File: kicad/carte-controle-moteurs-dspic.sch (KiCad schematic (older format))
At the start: 73 parts, among them P1 GND, P10 CONN_1, P11 ALIM, P12 MOTEUR 1, P13 MOTEUR 2, P14 PILES, P15 PILES, P17 I2C, P18 ENCODEUR 1, P19 ENCODEUR 2, P2 5V, P20 PROG, P21 Fixe, P22 Fixe, P23 Fixe, P24 Fixe, P3 3.3V, P4 EN, P5 L1, P6 H1, P7 L2, P8 H2, P9 CONN_1, U1 DSPIC33FJ, U2 L298_PAI225, U3 LM1117-3.3, X1 10 MHz

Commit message: Mise à jour des fichiers pour la nouvelle version de KiCAD
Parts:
- removed C10: 17p, symbol C
- removed C11, C12, C13: 1u, symbol CAPAPOL
- removed C14: 4.7u, symbol CAPAPOL
- removed C2, C3, C4: 100n, symbol C
- removed C6, C7, C8: 100u, symbol CAPAPOL
- removed D1, D10, D2, D3, D4, D5, D6, D7, D8, D9: 5A, symbol DIODE
- removed D11, D12: GREEN, symbol LED
- removed D13: RED, symbol LED
- removed D14, D15, D16, D17, D18, D19: ZENER, symbol DIODE
- removed P1: GND, symbol CONN_1
- removed P10, P9: CONN_1, symbol CONN_1
- removed P11: ALIM, symbol CONN_2
- removed P12: MOTEUR 1, symbol CONN_2
- removed P13: MOTEUR 2, symbol CONN_2
- removed P14, P15: PILES, symbol CONN_2
- removed P17: I2C, symbol CONN_4
- removed P18: ENCODEUR 1, symbol CONN_5
- removed P19: ENCODEUR 2, symbol CONN_5
- removed P2: 5V, symbol CONN_1
- removed P20: PROG, symbol CONN_5X2
- removed P21, P22, P23, P24: Fixe, symbol CONN_1
- removed P3: 3.3V, symbol CONN_1
- removed P4: EN, symbol CONN_1
- removed P5: L1, symbol CONN_1
- removed P6: H1, symbol CONN_1
- removed P7: L2, symbol CONN_1
- removed P8: H2, symbol CONN_1
- removed U3: LM1117-3.3, symbol LM317T
- removed X1: 10 MHz, symbol CRYSTAL
- added C10, C2, C3, C4, C7: 100u, Capacitors_THT:CP_Radial_D10.0mm_P2.50mm_P5.00mm, symbol CP
- added C11, C12: 17p, Capacitors_THT:C_Rect_L7.0mm_W3.5mm_P2.50mm_P5.00mm, symbol C
- added C13: 1u, Capacitors_THT:CP_Radial_D10.0mm_P2.50mm_P5.00mm, symbol CP
- added C14: 4.7u, Capacitors_THT:CP_Radial_D10.0mm_P2.50mm_P5.00mm, symbol CP
- added C6, C8: 100n, Capacitors_THT:C_Rect_L7.0mm_W3.5mm_P2.50mm_P5.00mm, symbol C
- added D1: RED, LEDs:LED_D3.0mm, symbol LED
- added D10, D11, D12, D3, D4, D5, D6, D7, D8, D9: 5A, Diodes_THT:D_A-405_P10.16mm_Horizontal, symbol D
- added D13, D14, D15, D16, D17, D18: 3A, Diodes_THT:D_A-405_P10.16mm_Horizontal, symbol D_Zener
- added D19: GREEN, LEDs:LED_D3.0mm, symbol LED
- added D2: ORANGE, LEDs:LED_D3.0mm, symbol LED
- added J1: PDB, Measurement_Points:Measurement_Point_Round-TH_Small, symbol Conn_01x01
- added J10: PWR_IN, Connectors_Molex:Molex_MiniFit-JR-5569-04A2_2x02x4.20mm_Angled, symbol Conn_02x02_Odd_Even
- added J11: GND, Measurement_Points:Measurement_Point_Round-TH_Small, symbol Conn_01x01
- added J12: 5V, Measurement_Points:Measurement_Point_Round-TH_Small, symbol Conn_01x01
- added J13: 3.3V, Measurement_Points:Measurement_Point_Round-TH_Small, symbol Conn_01x01
- added J14: EN, Measurement_Points:Measurement_Point_Round-TH_Small, symbol Conn_01x01
- added J15: MOTEUR 1, epsa_connect:KK_2C, symbol Conn_01x02
- added J16: MOTEUR 2, epsa_connect:KK_2C, symbol Conn_01x02
- added J17: L1, Measurement_Points:Measurement_Point_Round-TH_Small, symbol Conn_01x01
- added J18: H1, Measurement_Points:Measurement_Point_Round-TH_Small, symbol Conn_01x01
- added J19: L2, Measurement_Points:Measurement_Point_Round-TH_Small, symbol Conn_01x01
- added J2: I2C, epsa_connect:KK_4C, symbol Conn_01x04
- added J20: H2, Measurement_Points:Measurement_Point_Round-TH_Small, symbol Conn_01x01
- added J21: ENCODEUR 1, Pin_Headers:Pin_Header_Angled_1x05_Pitch2.54mm, symbol Conn_01x05
- added J22: RA1, Measurement_Points:Measurement_Point_Round-TH_Small, symbol Conn_01x01
- added J23: ENCODEUR 2, Pin_Headers:Pin_Header_Angled_1x05_Pitch2.54mm, symbol Conn_01x05
- added J3: PROG, Pin_Headers:Pin_Header_Angled_2x05_Pitch2.54mm, symbol Conn_02x05_Odd_Even
- added J4, J5: PILES, epsa_connect:KK_2C, symbol Conn_01x02
- added J6, J7, J8, J9: Fix, Connectors:1pin, symbol Conn_01x01
- added Y1: 10MHz, Crystals:Crystal_HC18-U_Vertical, symbol Crystal
- C1, C5: footprint (none) -> Capacitors_THT:C_Rect_L7.0mm_W3.5mm_P2.50mm_P5.00mm
- C9: value 17p -> 100n; footprint (none) -> Capacitors_THT:C_Rect_L7.0mm_W3.5mm_P2.50mm_P5.00mm
- R1, R12, R2, R5, R6, R7, R8: footprint (none) -> Resistors_THT:R_Axial_DIN0204_L3.6mm_D1.6mm_P2.54mm_Vertical
- R10, R11: value 470 -> 150; footprint (none) -> Resistors_THT:R_Axial_DIN0204_L3.6mm_D1.6mm_P2.54mm_Vertical
- R3: value 10 K -> 470; footprint (none) -> Resistors_THT:R_Axial_DIN0204_L3.6mm_D1.6mm_P2.54mm_Vertical
- R4: value 150 -> 470; footprint (none) -> Resistors_THT:R_Axial_DIN0204_L3.6mm_D1.6mm_P2.54mm_Vertical
- R9: value 150 -> 10K; footprint (none) -> Resistors_THT:R_Axial_DIN0204_L3.6mm_D1.6mm_P2.54mm_Vertical
- RR1: footprint (none) -> Resistors_THT:R_Array_SIP9
- U1: renamed from U2; footprint ANNEE 2017-2018 CONTACTER G. CHARREAUX -> TO_SOT_Packages_THT:Multiwatt-15_Vertical_StaggeredType1
- U2: renamed from U1; footprint (none) -> Housings_DIP:DIP-28_W7.62mm
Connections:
- net labels added: I2C_CLK, I2C_DATA, QEI1_CHA, QEI1_CHB, QEI2_CHA, QEI2_CHB
- net labels removed: I2C_clk, I2C_data, MCLR, QEI1_chA, QEI1_chB, QEI2_chA, QEI2_chB
- wire segments 179 -> 197
- no-connect marks 6 -> 7
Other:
- note added: "Connecteur d'alimentation"
- note added: "Convensions couleurs :\n1 - Noir : masse\n2 - Rouge : +5V\n3 - Orange : +3.3V\n4 - Jaune : BATT"
- note added: "DSPIC contrôle moteurs"
- note added: "Lissage tensions"
- note added: "Points de contrôle"
- note added: "Résistances de pull-up"
- note removed: "Branchement carte alim"
- note removed: "Connecteur I2C"
- note removed: "Connecteur de Programmation"
- note removed: "Conversion 5V-3.3V"
- note removed: "Dimensionner diodes (attention gros courant)"
- note removed: "Encodeurs moteurs"
- note removed: "Mettre infos en sérigraphie, pas en couche cuivre"
- note removed: "Need détrompeurs\nPlusieurs capas au lieu d'1 grosse"
- note removed: "PIC contrôle moteurs"
- note removed: "Pins de contrôle"
- note removed: "Pull up partagé i2c encodeur 20k réseau de résistance"
- note removed: "Rajouter diodes à endroits clés\n470 au lieu de 220"
- note removed: "Réseau de résistances - Pull up"
- note removed: "partir à la recherche de pdb"
- note removed: "pull up entre 10k et 100k en général 20k"
- note removed: "remplacer 18k par diodes zener"
- note removed: "vérifier si on a besoin du channel b des encodeurs (à priori non car ça sert pour la roue ibre)\nregrouper en1 et en2 (à voir)\nrb 10 et 11 utilisée pour debug (uart/rs232)"
- note removed: "zone à réserver sur le typon sans plan de masse pour puce d'identification"
- moved on the sheet: RR1, U1, U2

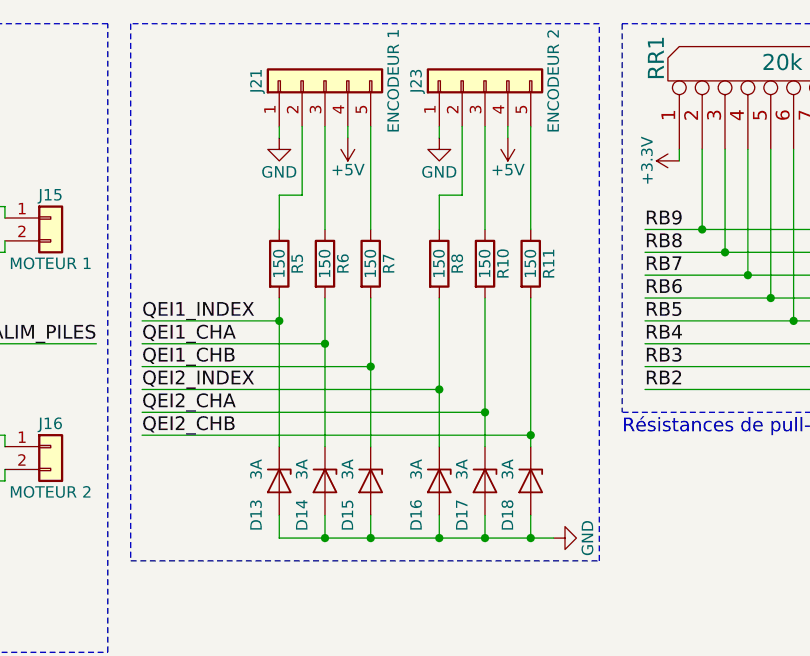
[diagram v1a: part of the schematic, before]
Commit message: Pré-validation CAO KiCAD
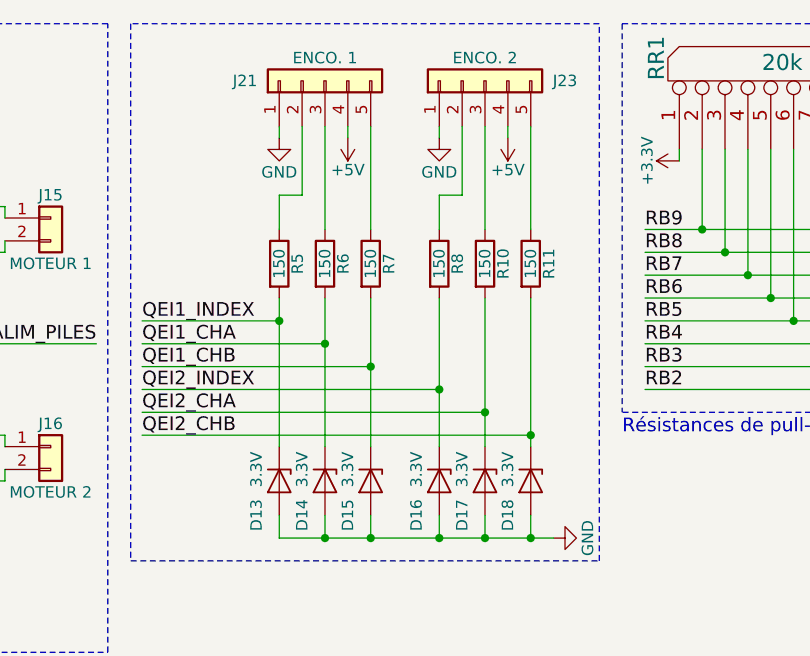
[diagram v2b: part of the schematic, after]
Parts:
- D13, D14, D15, D16, D17, D18: value 3A -> 3.3V
- J15, J16, J4, J5: footprint epsa_connect:KK_2C -> Connectors_Molex:Molex_MiniFit-JR-5569-02A2_2x01x4.20mm_Angled
- J21: value ENCODEUR 1 -> ENCO. 1
- J23: value ENCODEUR 2 -> ENCO. 2
- J3: footprint Pin_Headers:Pin_Header_Angled_2x05_Pitch2.54mm -> Pin_Headers:Pin_Header_Straight_2x05_Pitch2.54mm
- J6, J7, J8, J9: footprint Connectors:1pin -> Mounting_Holes:MountingHole_3.2mm_M3_Pad
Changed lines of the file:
@@
 Comp "Centrale Lyon"
 Comment1 ""
-Comment2 "Contacter G. CHARREAUX"
+Comment2 "Contacter G. CHARREAUX (chxguillaume@gmail.com)"
 Comment3 ""
 Comment4 ""
@@
 F 0 "J8" H 3300 5300 50  0000 C CNN
 F 1 "Fix" H 3300 5100 50  0000 C CNN
-F 2 "Connectors:1pin" H 3300 5200 50  0001 C CNN
+F 2 "Mounting_Holes:MountingHole_3.2mm_M3_Pad" H 3300 5200 50  0001 C CNN
 F 3 "" H 3300 5200 50  0001 C CNN
 	1    3300 5200
@@
 F 0 "J9" H 3300 5600 50  0000 C CNN
 F 1 "Fix" H 3300 5400 50  0000 C CNN
-F 2 "Connectors:1pin" H 3300 5500 50  0001 C CNN
+F 2 "Mounting_Holes:MountingHole_3.2mm_M3_Pad" H 3300 5500 50  0001 C CNN
 F 3 "" H 3300 5500 50  0001 C CNN
 	1    3300 5500
@@
 F 0 "J6" H 2950 5300 50  0000 C CNN
 F 1 "Fix" H 2950 5100 50  0000 C CNN
-F 2 "Connectors:1pin" H 2950 5200 50  0001 C CNN
+F 2 "Mounting_Holes:MountingHole_3.2mm_M3_Pad" H 2950 5200 50  0001 C CNN
 F 3 "" H 2950 5200 50  0001 C CNN
 	1    2950 5200
@@
 F 0 "J7" H 2950 5600 50  0000 C CNN
 F 1 "Fix" H 2950 5400 50  0000 C CNN
-F 2 "Connectors:1pin" H 2950 5500 50  0001 C CNN
+F 2 "Mounting_Holes:MountingHole_3.2mm_M3_Pad" H 2950 5500 50  0001 C CNN
 F 3 "" H 2950 5500 50  0001 C CNN
 	1    2950 5500
@@
 F 0 "J3" H 1800 4200 50  0000 C CNN
 F 1 "PROG" H 1800 3600 50  0000 C CNN
-F 2 "Pin_Headers:Pin_Header_Angled_2x05_Pitch2.54mm" H 1750 3900 50  0001 C CNN
+F 2 "Pin_Headers:Pin_Header_Straight_2x05_Pitch2.54mm" H 1750 3900 50  0001 C CNN
 F 3 "" H 1750 3900 50  0001 C CNN
 	1    1750 3900
@@
 F 0 "J15" H 4350 1600 50  0000 C CNN
 F 1 "MOTEUR 1" H 4350 1300 50  0000 C CNN
-F 2 "epsa_connect:KK_2C" H 4350 1500 50  0001 C CNN
+F 2 "Connectors_Molex:Molex_MiniFit-JR-5569-02A2_2x01x4.20mm_Angled" H 4350 1500 50  0001 C CNN
 F 3 "" H 4350 1500 50  0001 C CNN
 	1    4350 1500
@@
 F 0 "J16" H 4350 2600 50  0000 C CNN
 F 1 "MOTEUR 2" H 4350 2300 50  0000 C CNN
-F 2 "epsa_connect:KK_2C" H 4350 2500 50  0001 C CNN
+F 2 "Connectors_Molex:Molex_MiniFit-JR-5569-02A2_2x01x4.20mm_Angled" H 4350 2500 50  0001 C CNN
 F 3 "" H 4350 2500 50  0001 C CNN
 	1    4350 2500
@@
 P 5350 2650
 F 0 "D13" H 5500 2550 50  0000 C CNN
-F 1 "3A" H 5300 2550 50  0000 C CNN
+F 1 "3.3V" H 5300 2550 50  0000 C CNN
 F 2 "Diodes_THT:D_A-405_P10.16mm_Horizontal" H 5350 2650 50  0001 C CNN
 F 3 "" H 5350 2650 50  0001 C CNN
@@
 U 1 1 5A82BD44
 P 6250 900
-F 0 "J23" H 6250 1200 50  0000 C CNN
-F 1 "ENCODEUR 2" H 6250 600 50  0000 C CNN
+F 0 "J23" V 6250 550 50  0000 C CNN
+F 1 "ENCO. 2" V 6350 900 50  0000 C CNN
 F 2 "Pin_Headers:Pin_Header_Angled_1x05_Pitch2.54mm" H 6250 900 50  0001 C CNN
 F 3 "" H 6250 900 50  0001 C CNN
@@
 U 1 1 5A82F3E1
 P 5550 900
-F 0 "J21" H 5550 1200 50  0000 C CNN
-F 1 "ENCODEUR 1" H 5550 600 50  0000 C CNN
+F 0 "J21" V 5550 1250 50  0000 C CNN
+F 1 "ENCO. 1" V 5650 900 50  0000 C CNN
 F 2 "Pin_Headers:Pin_Header_Angled_1x05_Pitch2.54mm" H 5550 900 50  0001 C CNN
 F 3 "" H 5550 900 50  0001 C CNN
@@
 P 5550 2650
 F 0 "D14" H 5700 2550 50  0000 C CNN
-F 1 "3A" H 5500 2550 50  0000 C CNN
+F 1 "3.3V" H 5500 2550 50  0000 C CNN
 F 2 "Diodes_THT:D_A-405_P10.16mm_Horizontal" H 5550 2650 50  0001 C CNN
 F 3 "" H 5550 2650 50  0001 C CNN
@@
 P 5750 2650
 F 0 "D15" H 5900 2550 50  0000 C CNN
-F 1 "3A" H 5700 2550 50  0000 C CNN
+F 1 "3.3V" H 5700 2550 50  0000 C CNN
 F 2 "Diodes_THT:D_A-405_P10.16mm_Horizontal" H 5750 2650 50  0001 C CNN
 F 3 "" H 5750 2650 50  0001 C CNN
@@
 P 6050 2650
 F 0 "D16" H 6200 2550 50  0000 C CNN
-F 1 "3A" H 6000 2550 50  0000 C CNN
+F 1 "3.3V" H 6000 2550 50  0000 C CNN
 F 2 "Diodes_THT:D_A-405_P10.16mm_Horizontal" H 6050 2650 50  0001 C CNN
 F 3 "" H 6050 2650 50  0001 C CNN
@@
 P 6250 2650
 F 0 "D17" H 6400 2550 50  0000 C CNN
-F 1 "3A" H 6200 2550 50  0000 C CNN
+F 1 "3.3V" H 6200 2550 50  0000 C CNN
 F 2 "Diodes_THT:D_A-405_P10.16mm_Horizontal" H 6250 2650 50  0001 C CNN
 F 3 "" H 6250 2650 50  0001 C CNN
@@
 P 6450 2650
 F 0 "D18" H 6600 2550 50  0000 C CNN
-F 1 "3A" H 6400 2550 50  0000 C CNN
+F 1 "3.3V" H 6400 2550 50  0000 C CNN
 F 2 "Diodes_THT:D_A-405_P10.16mm_Horizontal" H 6450 2650 50  0001 C CNN
 F 3 "" H 6450 2650 50  0001 C CNN
@@
 F 0 "J4" H 2550 6350 50  0000 C CNN
 F 1 "PILES" H 2550 6050 50  0000 C CNN
-F 2 "epsa_connect:KK_2C" H 2550 6250 50  0001 C CNN
+F 2 "Connectors_Molex:Molex_MiniFit-JR-5569-02A2_2x01x4.20mm_Angled" H 2550 6250 50  0001 C CNN
 F 3 "" H 2550 6250 50  0001 C CNN
 	1    2550 6250
@@
 F 0 "J5" H 2550 6750 50  0000 C CNN
 F 1 "PILES" H 2550 6450 50  0000 C CNN
-F 2 "epsa_connect:KK_2C" H 2550 6650 50  0001 C CNN
+F 2 "Connectors_Molex:Molex_MiniFit-JR-5569-02A2_2x01x4.20mm_Angled" H 2550 6650 50  0001 C CNN
 F 3 "" H 2550 6650 50  0001 C CNN
 	1    2550 6650

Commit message: Changement empreintes résistances
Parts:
- R1, R10, R11, R12, R2, R3, R4, R5, R6, R7, R8, R9: footprint Resistors_THT:R_Axial_DIN0204_L3.6mm_D1.6mm_P2.54mm_Vertical -> Resistors_THT:R_Axial_DIN0204_L3.6mm_D1.6mm_P7.62mm_Horizontal
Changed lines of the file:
@@
 F 0 "R3" V 2130 4550 50  0000 C CNN
 F 1 "470" V 2050 4550 50  0000 C CNN
-F 2 "Resistors_THT:R_Axial_DIN0204_L3.6mm_D1.6mm_P2.54mm_Vertical" V 1980 4550 50  0001 C CNN
+F 2 "Resistors_THT:R_Axial_DIN0204_L3.6mm_D1.6mm_P7.62mm_Horizontal" V 1980 4550 50  0001 C CNN
 F 3 "" H 2050 4550 50  0001 C CNN
 	1    2050 4550
@@
 F 0 "R4" V 2130 5150 50  0000 C CNN
 F 1 "470" V 2050 5150 50  0000 C CNN
-F 2 "Resistors_THT:R_Axial_DIN0204_L3.6mm_D1.6mm_P2.54mm_Vertical" V 1980 5150 50  0001 C CNN
+F 2 "Resistors_THT:R_Axial_DIN0204_L3.6mm_D1.6mm_P7.62mm_Horizontal" V 1980 5150 50  0001 C CNN
 F 3 "" H 2050 5150 50  0001 C CNN
 	1    2050 5150
@@
 F 0 "R1" V 1180 1900 50  0000 C CNN
 F 1 "0" V 1100 1900 50  0000 C CNN
-F 2 "Resistors_THT:R_Axial_DIN0204_L3.6mm_D1.6mm_P2.54mm_Vertical" V 1030 1900 50  0001 C CNN
+F 2 "Resistors_THT:R_Axial_DIN0204_L3.6mm_D1.6mm_P7.62mm_Horizontal" V 1030 1900 50  0001 C CNN
 F 3 "" H 1100 1900 50  0001 C CNN
 	1    1100 1900
@@
 F 0 "R2" V 1180 2200 50  0000 C CNN
 F 1 "0" V 1100 2200 50  0000 C CNN
-F 2 "Resistors_THT:R_Axial_DIN0204_L3.6mm_D1.6mm_P2.54mm_Vertical" V 1030 2200 50  0001 C CNN
+F 2 "Resistors_THT:R_Axial_DIN0204_L3.6mm_D1.6mm_P7.62mm_Horizontal" V 1030 2200 50  0001 C CNN
 F 3 "" H 1100 2200 50  0001 C CNN
 	1    1100 2200
@@
 F 0 "R5" V 5430 1700 50  0000 C CNN
 F 1 "150" V 5350 1700 50  0000 C CNN
-F 2 "Resistors_THT:R_Axial_DIN0204_L3.6mm_D1.6mm_P2.54mm_Vertical" V 5280 1700 50  0001 C CNN
+F 2 "Resistors_THT:R_Axial_DIN0204_L3.6mm_D1.6mm_P7.62mm_Horizontal" V 5280 1700 50  0001 C CNN
 F 3 "" H 5350 1700 50  0001 C CNN
 	1    5350 1700
@@
 F 0 "R6" V 5630 1700 50  0000 C CNN
 F 1 "150" V 5550 1700 50  0000 C CNN
-F 2 "Resistors_THT:R_Axial_DIN0204_L3.6mm_D1.6mm_P2.54mm_Vertical" V 5480 1700 50  0001 C CNN
+F 2 "Resistors_THT:R_Axial_DIN0204_L3.6mm_D1.6mm_P7.62mm_Horizontal" V 5480 1700 50  0001 C CNN
 F 3 "" H 5550 1700 50  0001 C CNN
 	1    5550 1700
@@
 F 0 "R7" V 5830 1700 50  0000 C CNN
 F 1 "150" V 5750 1700 50  0000 C CNN
-F 2 "Resistors_THT:R_Axial_DIN0204_L3.6mm_D1.6mm_P2.54mm_Vertical" V 5680 1700 50  0001 C CNN
+F 2 "Resistors_THT:R_Axial_DIN0204_L3.6mm_D1.6mm_P7.62mm_Horizontal" V 5680 1700 50  0001 C CNN
 F 3 "" H 5750 1700 50  0001 C CNN
 	1    5750 1700
@@
 F 0 "R8" V 6130 1700 50  0000 C CNN
 F 1 "150" V 6050 1700 50  0000 C CNN
-F 2 "Resistors_THT:R_Axial_DIN0204_L3.6mm_D1.6mm_P2.54mm_Vertical" V 5980 1700 50  0001 C CNN
+F 2 "Resistors_THT:R_Axial_DIN0204_L3.6mm_D1.6mm_P7.62mm_Horizontal" V 5980 1700 50  0001 C CNN
 F 3 "" H 6050 1700 50  0001 C CNN
 	1    6050 1700
@@
 F 0 "R10" V 6330 1700 50  0000 C CNN
 F 1 "150" V 6250 1700 50  0000 C CNN
-F 2 "Resistors_THT:R_Axial_DIN0204_L3.6mm_D1.6mm_P2.54mm_Vertical" V 6180 1700 50  0001 C CNN
+F 2 "Resistors_THT:R_Axial_DIN0204_L3.6mm_D1.6mm_P7.62mm_Horizontal" V 6180 1700 50  0001 C CNN
 F 3 "" H 6250 1700 50  0001 C CNN
 	1    6250 1700
@@
 F 0 "R11" V 6530 1700 50  0000 C CNN
 F 1 "150" V 6450 1700 50  0000 C CNN
-F 2 "Resistors_THT:R_Axial_DIN0204_L3.6mm_D1.6mm_P2.54mm_Vertical" V 6380 1700 50  0001 C CNN
+F 2 "Resistors_THT:R_Axial_DIN0204_L3.6mm_D1.6mm_P7.62mm_Horizontal" V 6380 1700 50  0001 C CNN
 F 3 "" H 6450 1700 50  0001 C CNN
 	1    6450 1700
@@
 F 0 "R12" V 8430 5050 50  0000 C CNN
 F 1 "470" V 8350 5050 50  0000 C CNN
-F 2 "Resistors_THT:R_Axial_DIN0204_L3.6mm_D1.6mm_P2.54mm_Vertical" V 8280 5050 50  0001 C CNN
+F 2 "Resistors_THT:R_Axial_DIN0204_L3.6mm_D1.6mm_P7.62mm_Horizontal" V 8280 5050 50  0001 C CNN
 F 3 "" H 8350 5050 50  0001 C CNN
 	1    8350 5050
@@
 F 0 "R9" V 6000 3650 50  0000 C CNN
 F 1 "10K" V 6100 3650 50  0000 C CNN
-F 2 "Resistors_THT:R_Axial_DIN0204_L3.6mm_D1.6mm_P2.54mm_Vertical" V 6030 3650 50  0001 C CNN
+F 2 "Resistors_THT:R_Axial_DIN0204_L3.6mm_D1.6mm_P7.62mm_Horizontal" V 6030 3650 50  0001 C CNN
 F 3 "" H 6100 3650 50  0001 C CNN
 	1    6100 3650
